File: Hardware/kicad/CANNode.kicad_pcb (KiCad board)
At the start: 4 copper layers, 66 x 57.5 mm, 53 parts, among them J1 Conn_01x04, J11 Conn_01x04, J12 Conn_01x04, J2 Conn_01x04, J21 Conn_01x04, J31 Conn_01x04, J41 Conn_01x04, J42 Conn_01x04, J43 Conn_01x04, J44 Conn_01x04, J51 Conn_01x02, J61 Conn_02x04_Odd_Even, J81 Conn_01x10, J91 Conn_01x04, U1 Teensy3.2, U2 SN65HVD230, U21 PCA9306, U31 MAX3485, U41 MAX3485, U91 LM1117-5.0

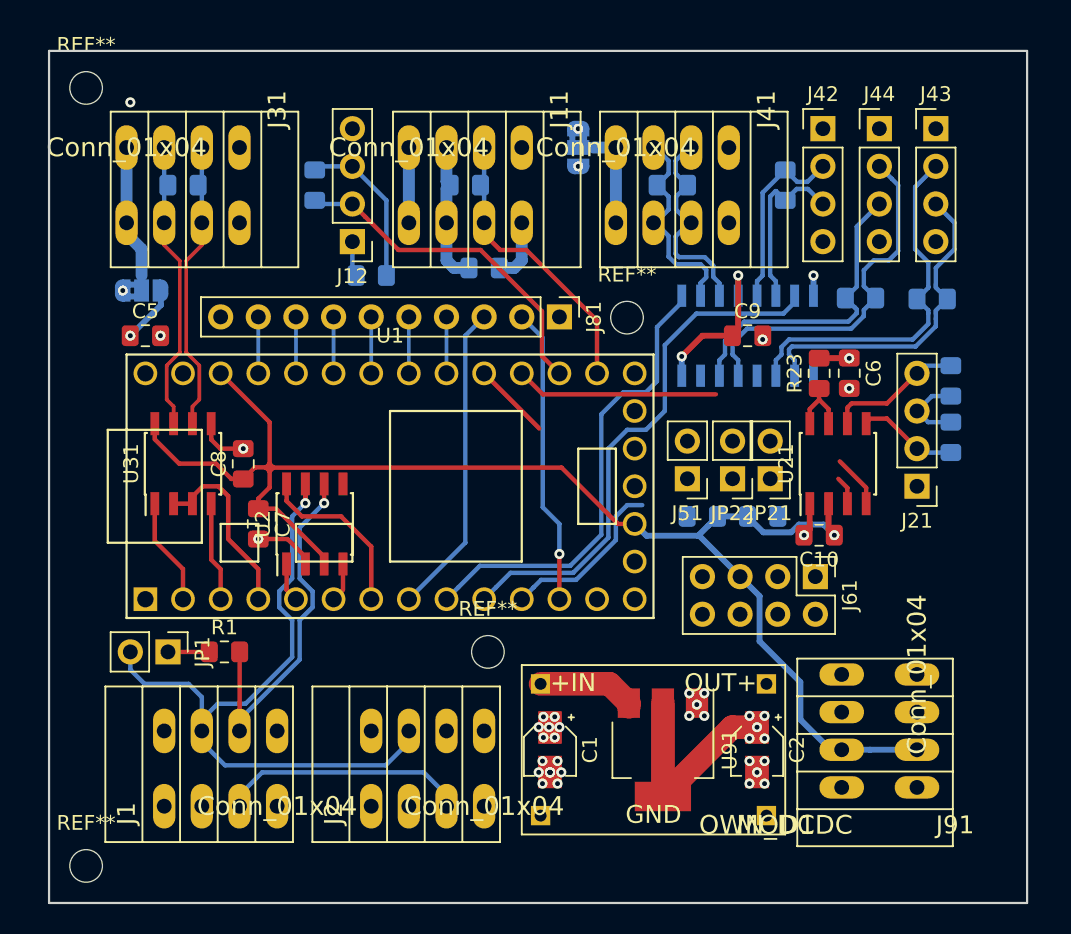
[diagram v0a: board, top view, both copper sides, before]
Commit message: looks good
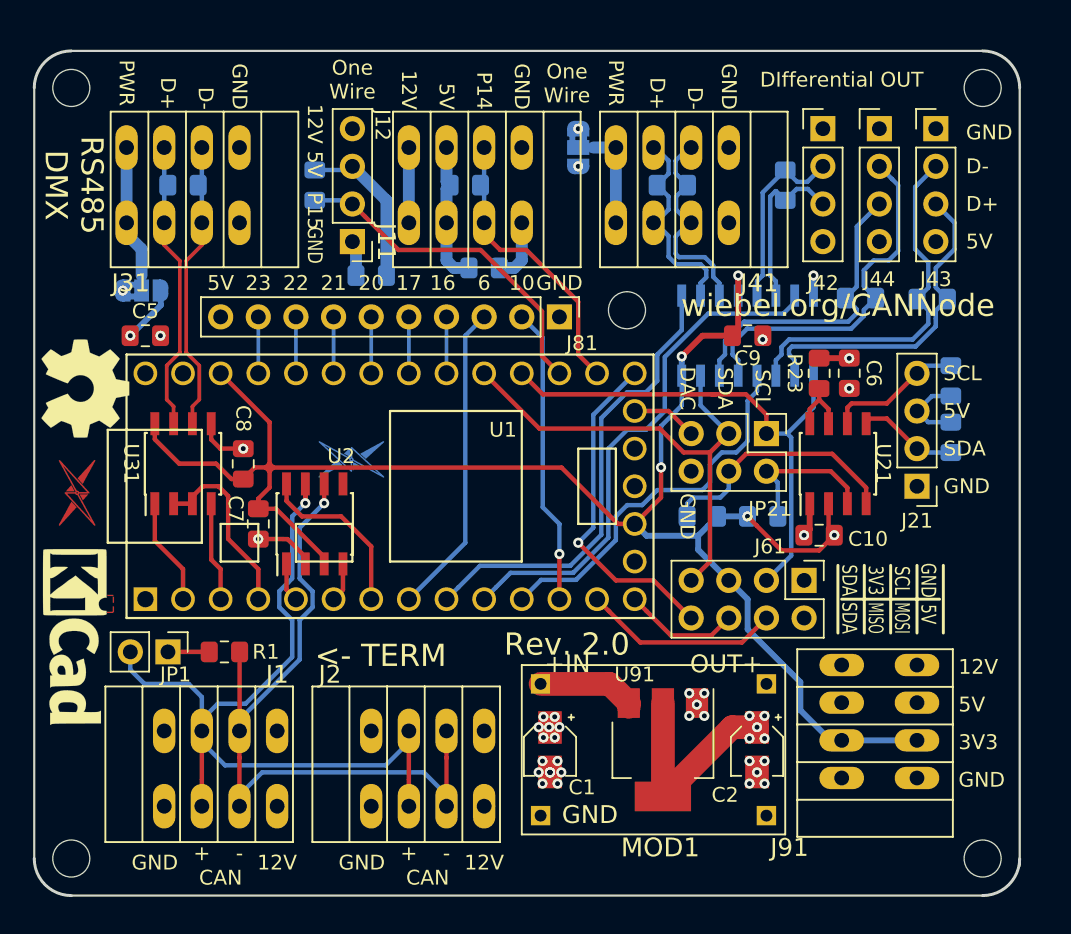
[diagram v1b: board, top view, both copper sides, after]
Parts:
- removed J51: Conn_01x02, Connector_PinHeader_2.54mm:PinHeader_1x02_P2.54mm_Vertical
- removed JP22: Jumper_NC_Small, Connector_PinHeader_2.54mm:PinHeader_1x02_P2.54mm_Vertical
- removed the REF** at (72.8, 91.7)
- removed the REF** at (109.3, 54.7)
- removed the REF** at (99.9, 77.2)
- removed the REF** at (72.8, 39.2)
- added ?: , own:LOGO_MID, F.Cu at (71.0, 64.3)
- added ?: , own:LOGO_MID, B.Cu at (88.5, 63.0)
- added REF**: MountingHole_2.5mm, MountingHole:MountingHole_2.5mm, F.Cu at (109.3, 54.2)
- added REF**: MountingHole_2.5mm, MountingHole:MountingHole_2.5mm, F.Cu at (71.8, 91.2)
- added REF**: MountingHole_2.5mm, MountingHole:MountingHole_2.5mm, F.Cu at (71.8, 39.2)
- added REF**: MountingHole_2.5mm, MountingHole:MountingHole_2.5mm, F.Cu at (133.3, 39.2)
- added REF**: MountingHole_2.5mm, MountingHole:MountingHole_2.5mm, F.Cu at (133.3, 91.2)
- added REF**: KiCAD Logo, Symbol:Symbol_KiCAD-Logo_CopperAndSilkScreenTop, F.Cu at (72.3, 76.2)
- added REF**: OSHW-Symbol_6.7x6mm_SilkScreen, Symbol:OSHW-Symbol_6.7x6mm_SilkScreen, F.Cu at (72.8, 59.4)
- JP21: value Jumper_NC_Small -> Conn_02x03_Odd_Even; footprint Connector_PinHeader_2.54mm:PinHeader_1x02_P2.54mm_Vertical -> Connector_PinHeader_2.54mm:PinHeader_2x03_P2.54mm_Vertical
- moved JP21 3.06 mm to (118.7, 62.5), turned to 270 degrees
- moved J61 0.80 mm to (121.3, 72.4)
- moved J91 0.63 mm to (128.9, 78.1)
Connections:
- J61 pad 7: Net-(J61-Pad7) -> /SDA0_17
- JP21 pad 1: Net-(JP21-Pad1) -> /SCL0_16
- JP21 pad 2: /SCL0_16 -> Net-(JP21-Pad2)
- R21 pad 1: Net-(JP21-Pad1) -> Net-(JP21-Pad2)
- R22 pad 1: Net-(JP22-Pad1) -> Net-(JP21-Pad4)
- U1 pad 19: Net-(J51-Pad2) -> Net-(JP21-Pad5)
- U1 pad 24: Net-(J61-Pad7) -> /SDA0_17
- U21 pad 3: Net-(JP21-Pad1) -> Net-(JP21-Pad2)
- U21 pad 4: Net-(JP22-Pad1) -> Net-(JP21-Pad4)
- U41 pad 15: Net-(J61-Pad7) -> /SDA0_17
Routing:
- net /SDA0_17: track 0.00 -> 33.1 mm
- net Net-(J61-Pad8): track 0.00 -> 22.7 mm, vias 0 -> 1
- net /SCL0_16: track 14.7 -> 35.8 mm
- net Net-(JP21-Pad4): track 0.00 -> 17.1 mm
- net /EN34_9: track 11.7 -> 26.0 mm
- net Net-(J61-Pad4): track 0.00 -> 13.3 mm
- net +3V3: track 107.5 -> 118.5 mm, vias 3 -> 5
- net +12V: track 128.2 -> 117.4 mm
- net Net-(JP21-Pad2): track 0.00 -> 10.4 mm
- net /CAN+: track 48.2 -> 58.3 mm
- net /CAN-: track 42.6 -> 52.8 mm
- net Net-(J61-Pad6): track 0.00 -> 7.85 mm
- net Net-(J61-Pad7): track 5.71 -> 0.00 mm
- net Net-(JP21-Pad5): track 0.00 -> 4.44 mm
- net Net-(JP22-Pad1): track 3.60 -> 0.00 mm
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- added copper zone on F.Cu, net (none)
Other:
- board size 66 x 57.5 mm -> 66.5 x 57 mm
- board text added: "+"
- board text added: "-"
- board text added: "10"
- board text added: "12V"
- board text added: "16"
- board text added: "17"
- board text added: "20"
- board text added: "21"
- board text added: "22"
- board text added: "23"
- board text added: "3V3"
- board text added: "5V"
- board text added: "6"
- board text added: "<- TERM"
- board text added: "CAN"
- board text added: "D+"
- board text added: "D-"
- board text added: "DAC"
- board text added: "DIfferential OUT"
- board text added: "GND"
- board text added: "MISO"
- board text added: "MOSI"
- board text added: "One Wire"
- board text added: "P14"
- board text added: "P15"
- board text added: "PWR"
- board text added: "RS485 DMX"
- board text added: "Rev. 2.0"
- board text added: "SCL"
- board text added: "SDA"
- board text added: "wiebel.org/CANNode"
